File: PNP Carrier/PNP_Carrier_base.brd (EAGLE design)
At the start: 90 x 104 mm, 0 parts

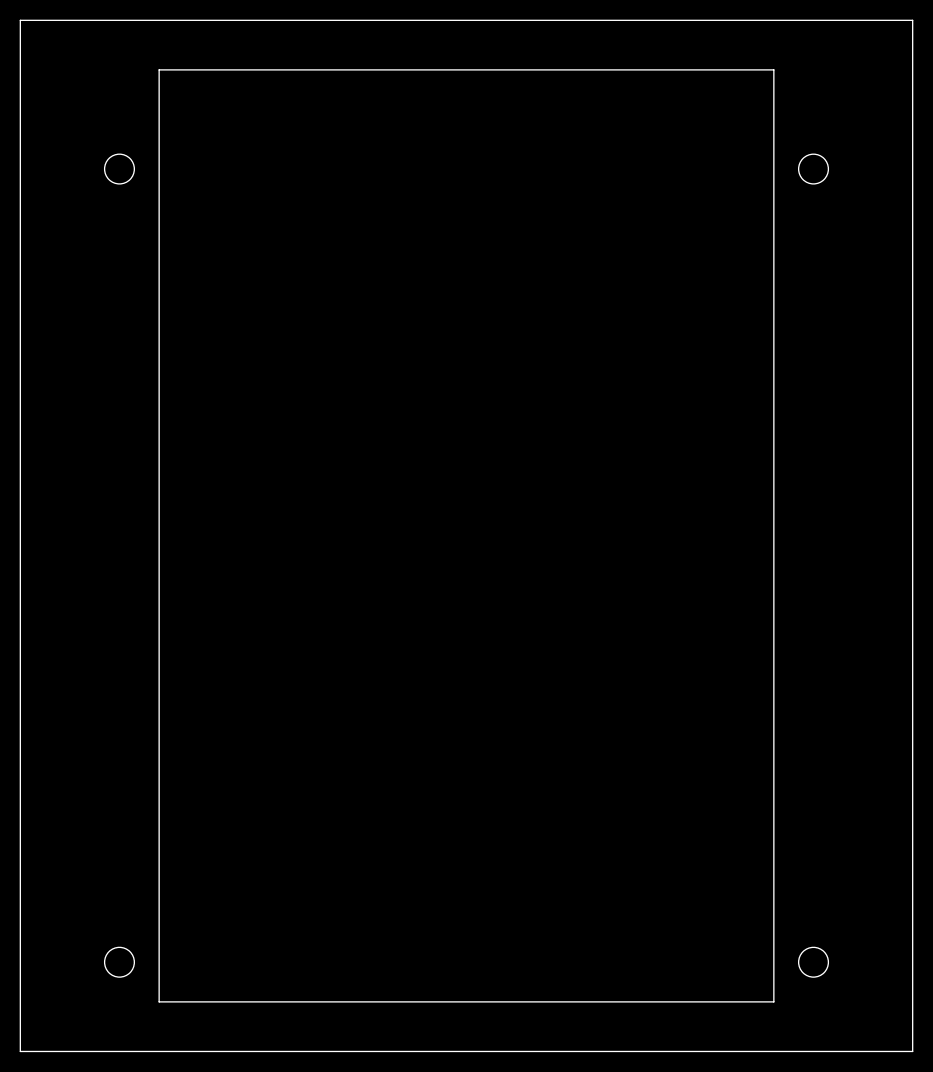
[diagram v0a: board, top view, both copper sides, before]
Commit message: Updated PNP Files
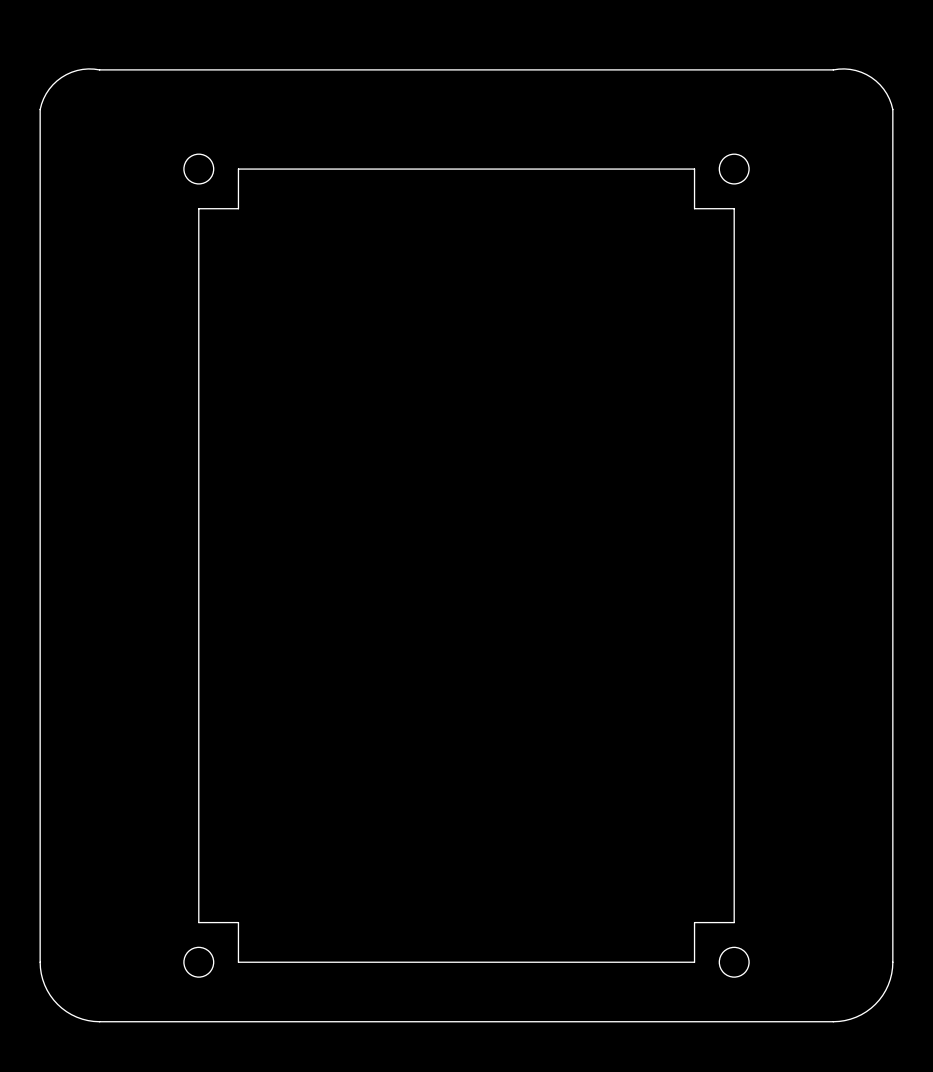
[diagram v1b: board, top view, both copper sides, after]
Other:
- board size 90 x 104 mm -> 86 x 96.1 mm
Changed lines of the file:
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@@
 <board>
 <plain>
-<wire x1="-15" y1="-6" x2="-15" y2="98" width="0.1016" layer="20"/>
-<wire x1="-15" y1="98" x2="75" y2="98" width="0.1016" layer="20"/>
-<wire x1="75" y1="98" x2="75" y2="-6" width="0.1016" layer="20"/>
-<wire x1="75" y1="-6" x2="-15" y2="-6" width="0.1016" layer="20"/>
-<wire x1="-1" y1="93" x2="61" y2="93" width="0.1016" layer="20"/>
-<wire x1="61" y1="93" x2="61" y2="-1" width="0.1016" layer="20"/>
-<wire x1="61" y1="-1" x2="-1" y2="-1" width="0.1016" layer="20"/>
-<wire x1="-1" y1="-1" x2="-1" y2="93" width="0.1016" layer="20"/>
-<hole x="-5" y="3" drill="3"/>
-<hole x="65" y="3" drill="3"/>
-<hole x="65" y="83" drill="3"/>
-<hole x="-5" y="83" drill="3"/>
+<hole x="3" y="3" drill="3"/>
+<hole x="57" y="3" drill="3"/>
+<hole x="57" y="83" drill="3"/>
+<hole x="3" y="83" drill="3"/>
+<wire x1="7" y1="3" x2="7" y2="7" width="0.01" layer="20"/>
+<wire x1="7" y1="7" x2="3" y2="7" width="0.01" layer="20"/>
+<wire x1="3" y1="7" x2="3" y2="79" width="0.01" layer="20"/>
+<wire x1="3" y1="79" x2="7" y2="79" width="0.01" layer="20"/>
+<wire x1="7" y1="79" x2="7" y2="83" width="0.01" layer="20"/>
+<wire x1="7" y1="83" x2="53" y2="83" width="0.01" layer="20"/>
+<wire x1="53" y1="83" x2="53" y2="79" width="0.01" layer="20"/>
+<wire x1="53" y1="79" x2="57" y2="79" width="0.01" layer="20"/>
+<wire x1="57" y1="79" x2="57" y2="7" width="0.01" layer="20"/>
+<wire x1="57" y1="7" x2="53" y2="7" width="0.01" layer="20"/>
+<wire x1="53" y1="7" x2="53" y2="3" width="0.01" layer="20"/>
+<wire x1="53" y1="3" x2="7" y2="3" width="0.01" layer="20"/>
+<wire x1="-13" y1="3" x2="-13" y2="89" width="0.01" layer="20"/>
+<wire x1="-7" y1="93" x2="67" y2="93" width="0.01" layer="20"/>
+<wire x1="73" y1="89" x2="73" y2="3" width="0.01" layer="20"/>
+<wire x1="67" y1="-3" x2="-7" y2="-3" width="0.01" layer="20"/>
+<wire x1="-13" y1="89" x2="-7" y2="93" width="0.01" layer="20" curve="-90"/>
+<wire x1="73" y1="89" x2="67" y2="93" width="0.01" layer="20" curve="90"/>
+<wire x1="67" y1="-3" x2="73" y2="3" width="0.01" layer="20" curve="90"/>
+<wire x1="-7" y1="-3" x2="-13" y2="3" width="0.01" layer="20" curve="-90"/>
 </plain>
 <attributes>
